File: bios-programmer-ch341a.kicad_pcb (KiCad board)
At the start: 2 copper layers, 50 x 56 mm, 28 parts, among them J1 USB_B_Micro, J4 +Banana+, J5 -Banana-, J6 ZIF16, J7 Conn_02x04_Counter_Clockwise, J8 Conn_02x04_Counter_Clockwise, SW1 RESET, U1 CH341A, U2 ISO6741, U3 ADuM1252, Y1 12M

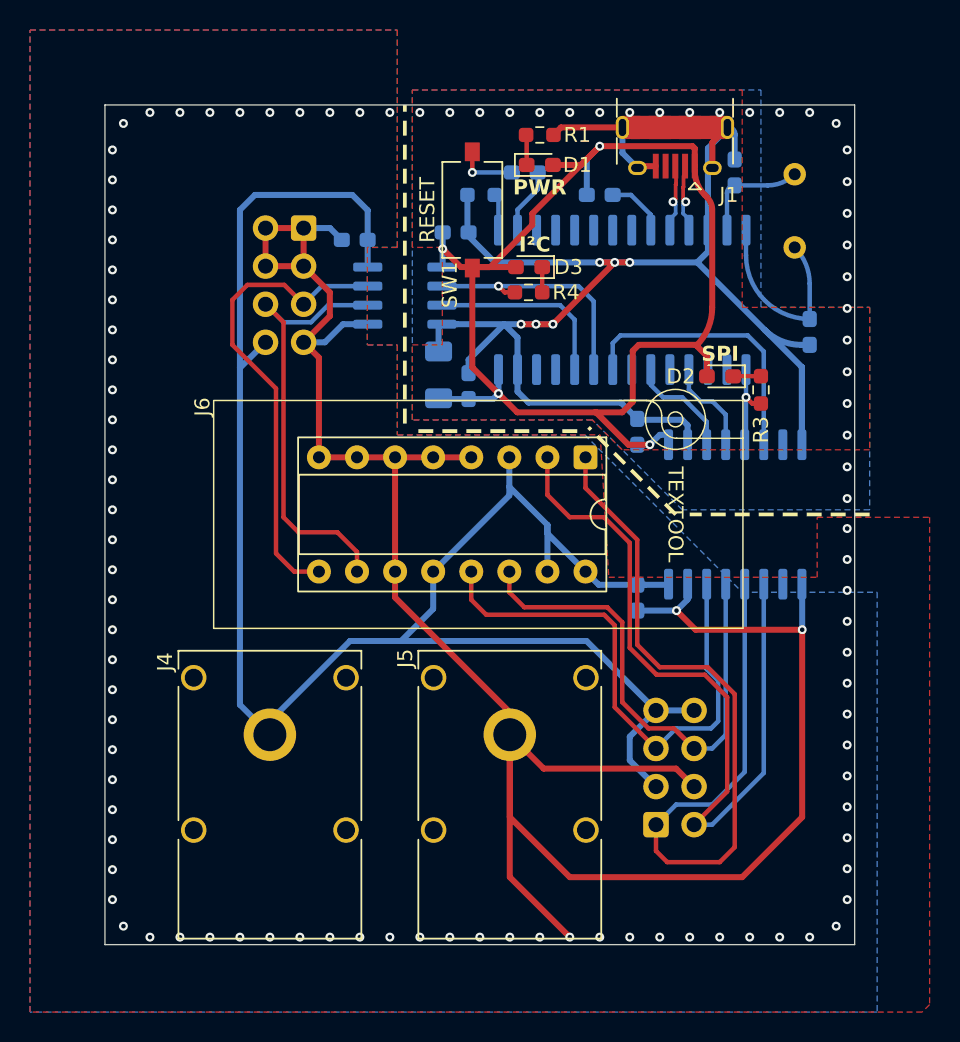
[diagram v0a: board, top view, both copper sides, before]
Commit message: PCB: so satisfying ... rounded some tracks just because I can :)
Yeah, I shouldn't ben doing this since it's strictly not necessary. But just
imagine all these electronics moving at light speed and then bumping again a
sharp corner! They might hurt themselves, possibly leading to a universe-ending
event. Or not.
Technically I'm pretty sure I read a application note or something about it
once, but I'm also pretty sure that all of this has happened before at least
once. So yeah, fun life, right?
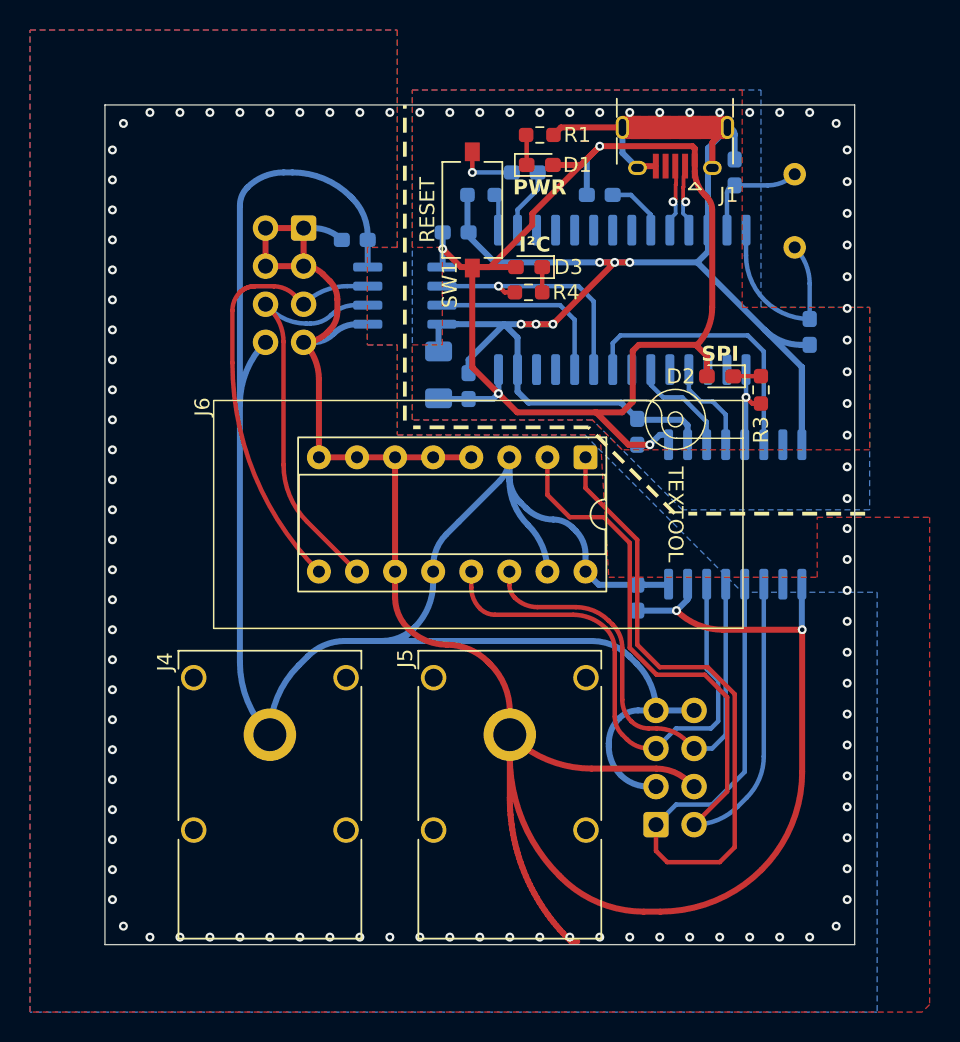
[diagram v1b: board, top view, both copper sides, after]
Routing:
- net VDD: track 122.8 -> 142.0 mm
- net /SCL_I: track 29.7 -> 27.0 mm
- net /CLK_I: track 34.6 -> 32.1 mm
- net /SDA_I: track 32.0 -> 30.6 mm
- net GNDD: track 442.6 -> 443.6 mm
